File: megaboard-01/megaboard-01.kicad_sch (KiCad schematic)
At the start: 10 parts, among them J1 Conn_01x01_Pin, J2 Conn_01x01_Pin, J3 Conn_01x03_Pin, J4 Conn_01x01_Pin, J5 Conn_01x01_Pin, U1 THS3091DDAR

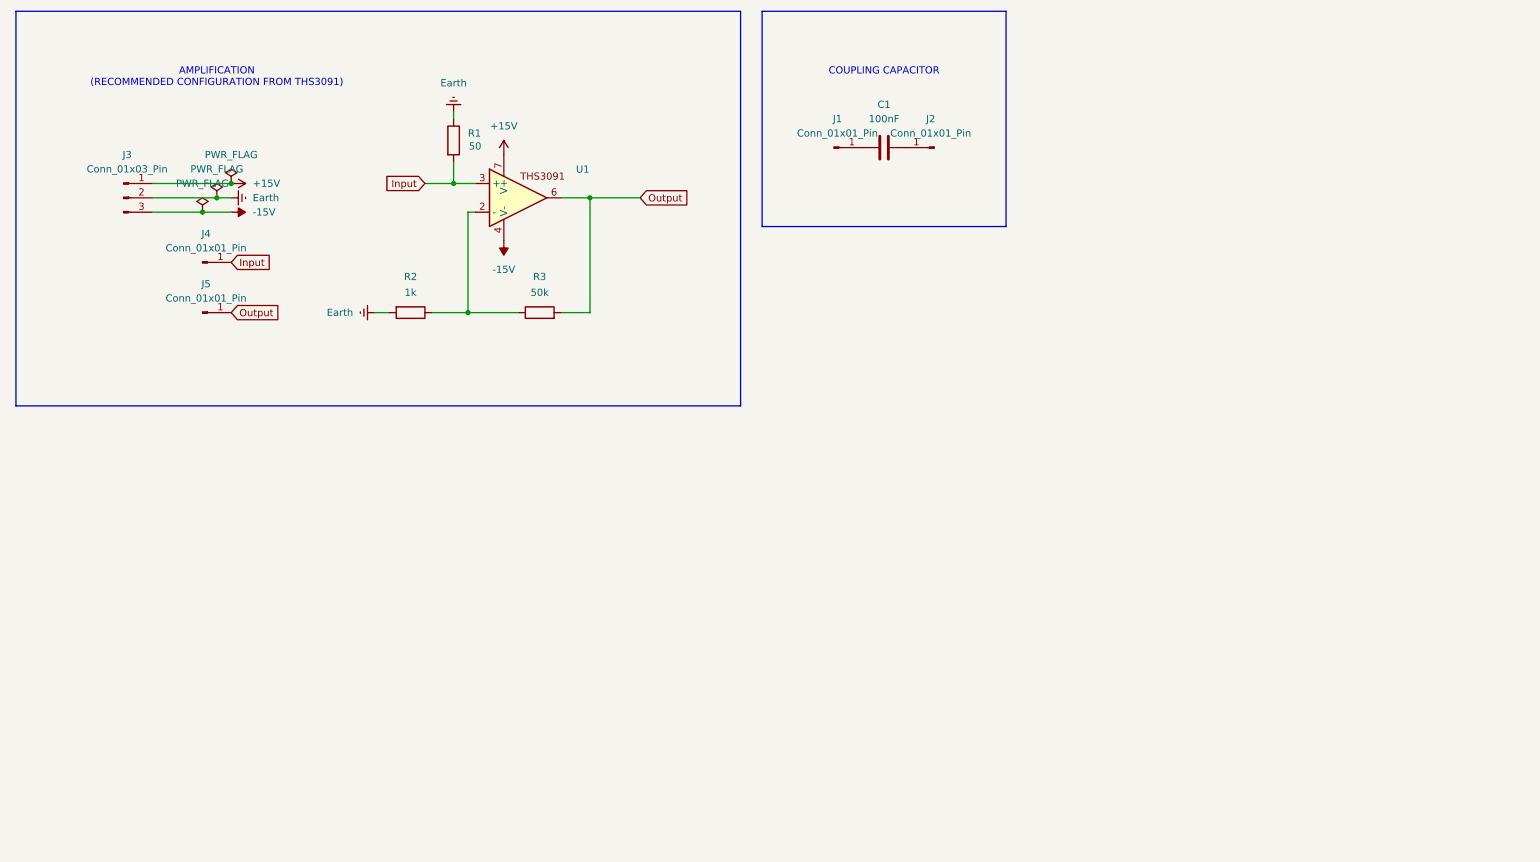
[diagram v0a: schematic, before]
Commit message: change megaboard
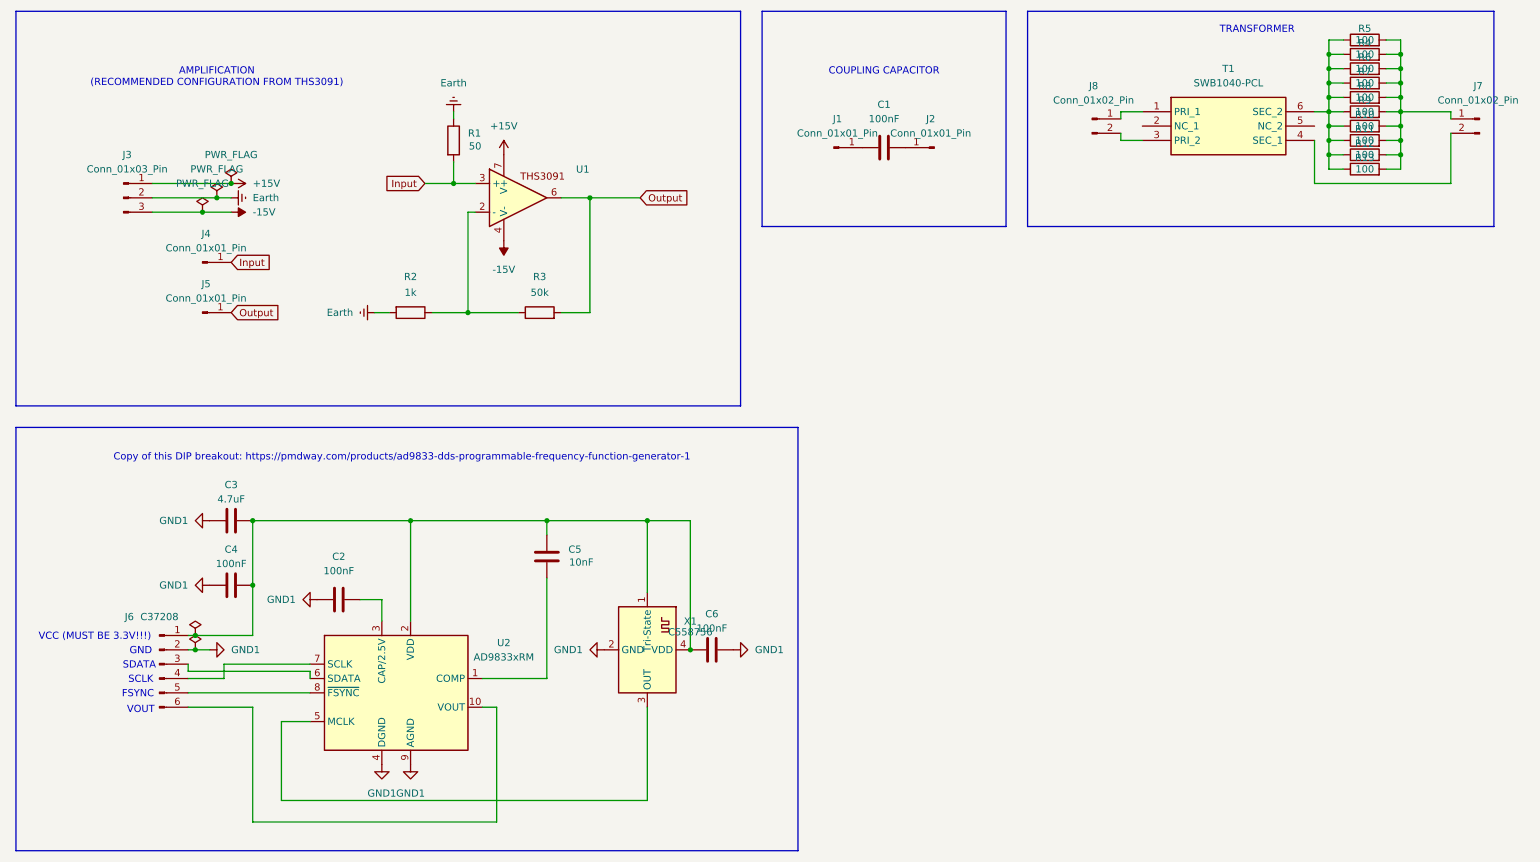
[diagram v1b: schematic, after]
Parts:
- added C2, C4, C6: C14663, Capacitor_SMD:C_0603_1608Metric, symbol Device:C
- added C3: C1779, Capacitor_SMD:C_0805_2012Metric, symbol Device:C
- added C5: C57112, Capacitor_SMD:C_0603_1608Metric, symbol Device:C
- added J6: C37208, Connector_PinHeader_2.54mm:PinHeader_1x06_P2.54mm_Vertical, symbol Connector:Conn_01x06_Pin
- added J7, J8: Conn_01x02_Pin, Connector_PinHeader_2.54mm:PinHeader_1x02_P2.54mm_Vertical, symbol Connector:Conn_01x02_Pin
- added R10, R11, R12, R13, R4, R5, R6, R7, R8, R9: C17901, Resistor_SMD:R_1206_3216Metric, symbol Device:R
- added T1: SWB1040-PCL, Mouser:SWB1040PCL, symbol SWB1040-PCL:SWB1040-PCL
- added U2: AD9833xRM, Package_SO:MSOP-10_3x3mm_P0.5mm, symbol Interface:AD9833xRM
- added X1: C558756, Crystal:Crystal_SMD_7050-4Pin_7.0x5.0mm, symbol LouisCustom:OCETCLJANF
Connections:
- new net: C3.2, C4.2, C5.1, C6.1, J6.1 (Pin_1), U2.2 (VDD), X1.1 (Tri-State), X1.4 (VDD)
- new net: U2.5 (MCLK), X1.3 (OUT)
- new net: R10.1, R11.1, R12.1, R13.1, R4.1, R5.1, R6.1, R7.1, R8.1, R9.1, T1.6 (SEC_2)
- new net: J7.1 (Pin_1), R10.2, R11.2, R12.2, R13.2, R4.2, R5.2, R6.2, R7.2, R8.2, R9.2
- new net: J6.3 (Pin_3), U2.6 (SDATA)
- new net: J6.4 (Pin_4), U2.7 (SCLK)
- new net: J6.5 (Pin_5), U2.8 (~{FSYNC})
- new net: J6.6 (Pin_6), U2.10 (VOUT)
- new net: C5.2, U2.1 (COMP)
- new net: C2.2, U2.3 (CAP/2.5V)
- new net: J7.2 (Pin_2), T1.4 (SEC_1)
- new net: J8.1 (Pin_1), T1.1 (PRI_1)
- new net: J8.2 (Pin_2), T1.3 (PRI_2)
- new net GND1: C2.1, C3.1, C4.1, C6.2, J6.2 (Pin_2), U2.4 (DGND), U2.9 (AGND), X1.2 (GND)
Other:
- note added: "Copy of this DIP breakout: https://pmdway.com/products/ad9833-dds-programmable-frequency-function-generator-1"
- note added: "FSYNC"
- note added: "GND"
- note added: "SCLK"
- note added: "SDATA"
- note added: "TRANSFORMER"
- note added: "VCC (MUST BE 3.3V!!!)"
- note added: "VOUT"
